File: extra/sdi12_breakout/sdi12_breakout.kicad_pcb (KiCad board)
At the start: 2 copper layers, 69 x 69 mm, 8 parts, among them J1 Conn_01x03_Socket, J2 Conn_01x03_Socket, J3 Conn_01x03_Socket, J4 Conn_01x03_Socket, J5 AudioJack3, J6 AudioJack3, J7 AudioJack3, J8 AudioJack3

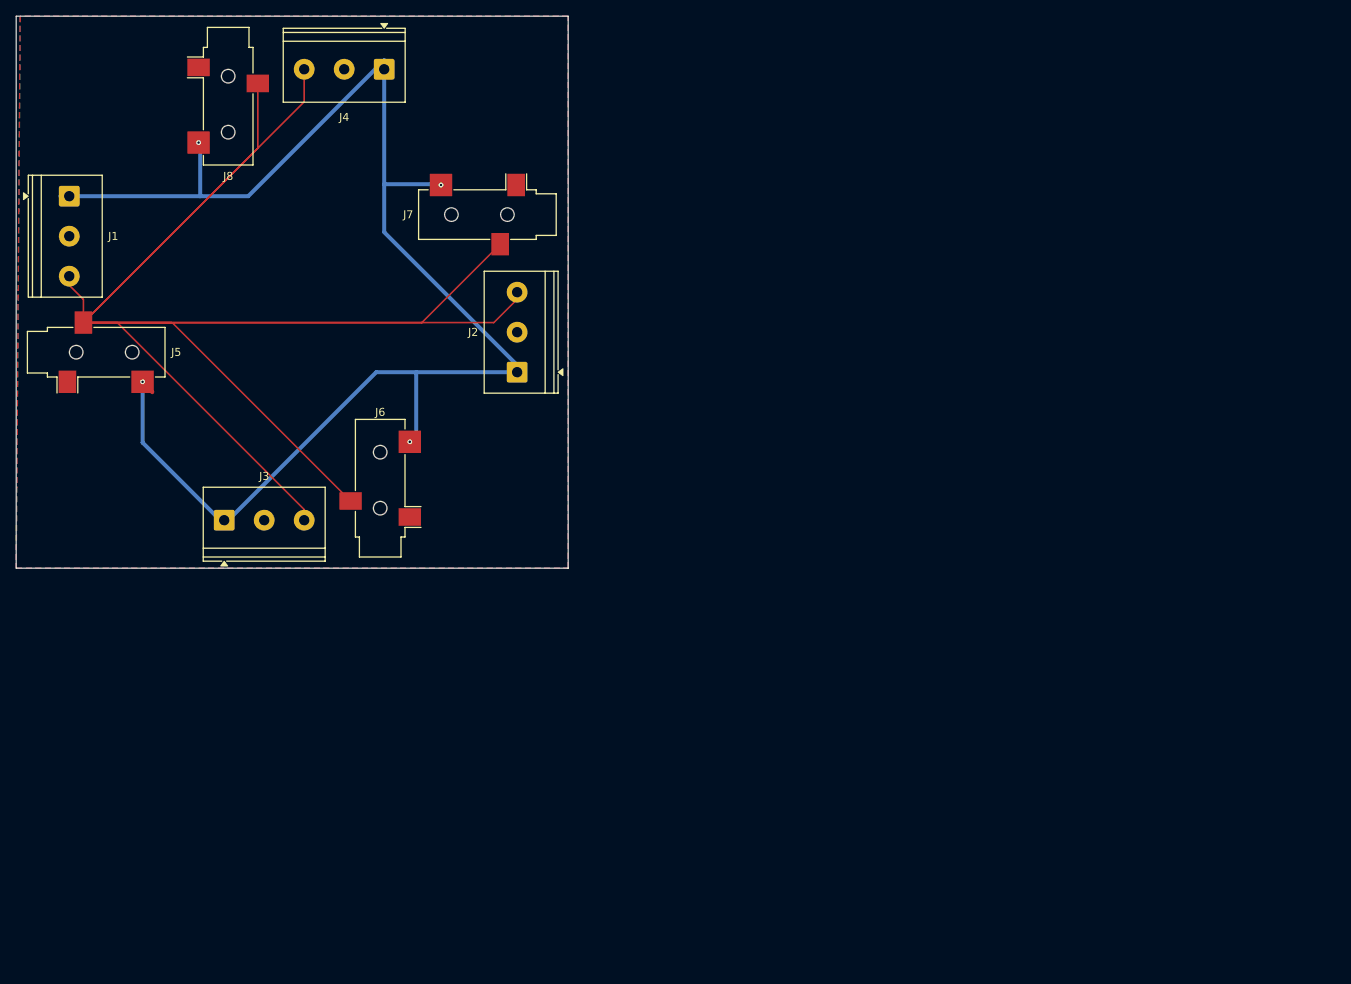
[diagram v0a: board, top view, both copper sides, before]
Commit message: Regenerated production file
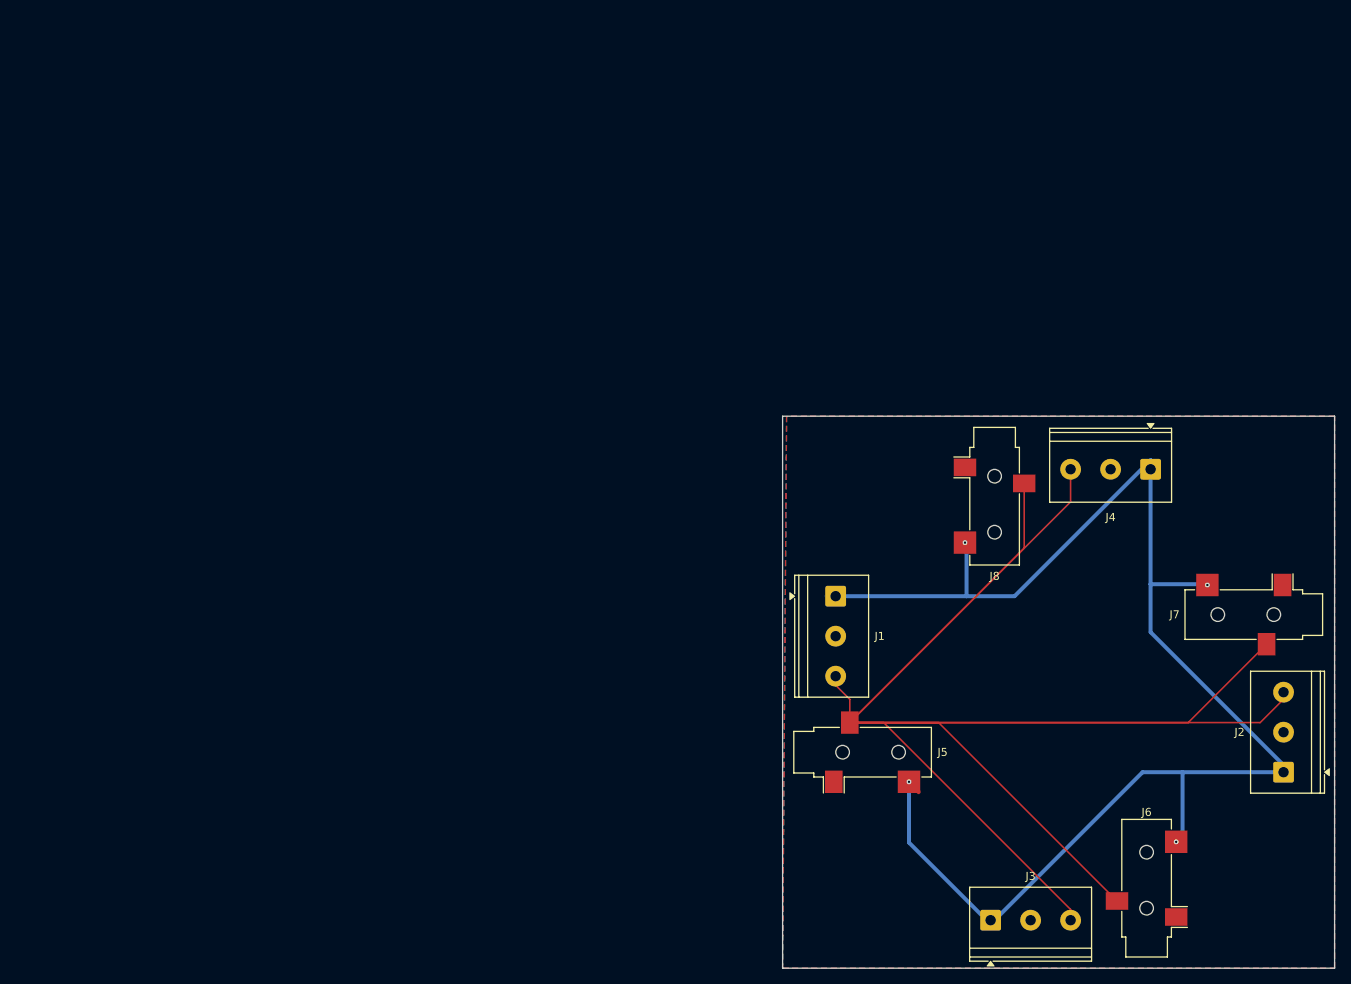
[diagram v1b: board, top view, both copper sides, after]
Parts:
- moved J1 108.1 mm to (114.9, 85.5)
- moved J3 108.1 mm to (134.3, 126.0)
- moved J4 108.1 mm to (154.3, 69.6)
- moved J6 108.1 mm to (153.8, 122.0)
- moved J8 108.1 mm to (134.8, 73.0)
- moved J5 108.1 mm to (118.3, 105.0)
- moved J2 108.1 mm to (170.9, 107.5)
- moved J7 108.1 mm to (167.2, 87.8)
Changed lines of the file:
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@@
 	(footprint "TerminalBlock_Phoenix:TerminalBlock_Phoenix_PT-1,5-3-5.0-H_1x03_P5.00mm_Horizontal"
 		(layer "F.Cu")
-		(at 75.1175 57.5 90)
+		(at 170.9175 107.5 90)
 		(descr "Terminal Block Phoenix PT-1,5-3-5.0-H, 3 pins, pitch 5mm, size 15x9mm, drill diameter 1.3mm, pad diameter 2.6mm, http://www.mouser.com/ds/2/324/ItemDetail_1935161-922578.pdf, script-generated using https://gitlab.com/kicad/libraries/kicad-footprint-generator/-/tree/master/scripts/TerminalBlock_Phoenix")
 		(tags "THT Terminal Block Phoenix PT-1,5-3-5.0-H pitch 5mm size 15x9mm drill 1.3mm pad 2.6mm")
@@
 	(footprint "TerminalBlock_Phoenix:TerminalBlock_Phoenix_PT-1,5-3-5.0-H_1x03_P5.00mm_Horizontal"
 		(layer "F.Cu")
-		(at 58.5 19.6325 180)
+		(at 154.3 69.6325 180)
 		(descr "Terminal Block Phoenix PT-1,5-3-5.0-H, 3 pins, pitch 5mm, size 15x9mm, drill diameter 1.3mm, pad diameter 2.6mm, http://www.mouser.com/ds/2/324/ItemDetail_1935161-922578.pdf, script-generated using https://gitlab.com/kicad/libraries/kicad-footprint-generator/-/tree/master/scripts/TerminalBlock_Phoenix")
 		(tags "THT Terminal Block Phoenix PT-1,5-3-5.0-H pitch 5mm size 15x9mm drill 1.3mm pad 2.6mm")
@@
 	(footprint "Connector_Audio:Jack_3.5mm_CUI_SJ-3523-SMT_Horizontal"
 		(layer "F.Cu")
-		(at 71.4 37.8 -90)
+		(at 167.2 87.8 -90)
 		(descr "3.5 mm, Stereo, Right Angle, Surface Mount (SMT), Audio Jack Connector (https://www.cui.com/product/resource/sj-352x-smt-series.pdf)")
 		(tags "3.5mm audio cui horizontal jack stereo")
@@
 	(footprint "Connector_Audio:Jack_3.5mm_CUI_SJ-3523-SMT_Horizontal"
 		(layer "F.Cu")
-		(at 22.5 55 90)
+		(at 118.3 105 90)
 		(descr "3.5 mm, Stereo, Right Angle, Surface Mount (SMT), Audio Jack Connector (https://www.cui.com/product/resource/sj-352x-smt-series.pdf)")
 		(tags "3.5mm audio cui horizontal jack stereo")
@@
 	(footprint "TerminalBlock_Phoenix:TerminalBlock_Phoenix_PT-1,5-3-5.0-H_1x03_P5.00mm_Horizontal"
 		(layer "F.Cu")
-		(at 38.5 76)
+		(at 134.3 126)
 		(descr "Terminal Block Phoenix PT-1,5-3-5.0-H, 3 pins, pitch 5mm, size 15x9mm, drill diameter 1.3mm, pad diameter 2.6mm, http://www.mouser.com/ds/2/324/ItemDetail_1935161-922578.pdf, script-generated using https://gitlab.com/kicad/libraries/kicad-footprint-generator/-/tree/master/scripts/TerminalBlock_Phoenix")
 		(tags "THT Terminal Block Phoenix PT-1,5-3-5.0-H pitch 5mm size 15x9mm drill 1.3mm pad 2.6mm")
@@
 	(footprint "Connector_Audio:Jack_3.5mm_CUI_SJ-3523-SMT_Horizontal"
 		(layer "F.Cu")
-		(at 58 72 180)
+		(at 153.8 122 180)
 		(descr "3.5 mm, Stereo, Right Angle, Surface Mount (SMT), Audio Jack Connector (https://www.cui.com/product/resource/sj-352x-smt-series.pdf)")
 		(tags "3.5mm audio cui horizontal jack stereo")
@@
 	(footprint "Connector_Audio:Jack_3.5mm_CUI_SJ-3523-SMT_Horizontal"
 		(layer "F.Cu")
-		(at 39 23)
+		(at 134.8 73)
 		(descr "3.5 mm, Stereo, Right Angle, Surface Mount (SMT), Audio Jack Connector (https://www.cui.com/product/resource/sj-352x-smt-series.pdf)")
 		(tags "3.5mm audio cui horizontal jack stereo")
@@
 	(footprint "TerminalBlock_Phoenix:TerminalBlock_Phoenix_PT-1,5-3-5.0-H_1x03_P5.00mm_Horizontal"
 		(layer "F.Cu")
-		(at 19.1325 35.5 -90)
+		(at 114.9325 85.5 -90)
 		(descr "Terminal Block Phoenix PT-1,5-3-5.0-H, 3 pins, pitch 5mm, size 15x9mm, drill diameter 1.3mm, pad diameter 2.6mm, http://www.mouser.com/ds/2/324/ItemDetail_1935161-922578.pdf, script-generated using https://gitlab.com/kicad/libraries/kicad-footprint-generator/-/tree/master/scripts/TerminalBlock_Phoenix")
 		(tags "THT Terminal Block Phoenix PT-1,5-3-5.0-H pitch 5mm size 15x9mm drill 1.3mm pad 2.6mm")
@@
 	)
 	(gr_rect
-		(start 12.5 13)
-		(end 81.5 82)
+		(start 108.3 63)
+		(end 177.3 132)
 		(stroke
 			(width 0.05)
@@
 	)
 	(gr_text "${TITLE}\n${COMPANY}\n${ISSUE_DATE}\n${REVISION}"
-		(at 56 50 0)
+		(at 151.8 100 0)
 		(layer "B.SilkS")
 		(effects
@@
 	)
 	(segment
-		(start 20.9 51.3)
-		(end 25.138477 51.3)
+		(start 116.7 101.3)
+		(end 120.938477 101.3)
 		(width 0.2)
 		(layer "F.Cu")
@@
 	)
 	(segment
-		(start 72.2 51.3)
-		(end 76 47.5)
+		(start 168 101.3)
+		(end 171.8 97.5)
 		(width 0.2)
 		(layer "F.Cu")
@@
 	)
 	(segment
-		(start 48.5 74.661523)
-		(end 48.5 76.5)
+		(start 144.3 124.661523)
+		(end 144.3 126.5)
 		(width 0.2)
 		(layer "F.Cu")
@@
 	)
 	(segment
-		(start 20.9 48.4)
-		(end 20.9 51.3)
+		(start 116.7 98.4)
+		(end 116.7 101.3)
 		(width 0.2)
 		(layer "F.Cu")
@@
 	)
 	(segment
-		(start 20.9 51.3)
-		(end 48.5 23.7)
+		(start 116.7 101.3)
+		(end 144.3 73.7)
 		(width 0.2)
 		(layer "F.Cu")
@@
 	)
 	(segment
-		(start 20.9 51.3)
-		(end 63.2 51.3)
+		(start 116.7 101.3)
+		(end 159 101.3)
 		(width 0.2)
 		(layer "F.Cu")
@@
 	)
 	(segment
-		(start 20.9 51.3)
-		(end 32 51.3)
+		(start 116.7 101.3)
+		(end 127.8 101.3)
 		(width 0.2)
 		(layer "F.Cu")
@@
 	)
 	(segment
-		(start 20.9 51.3)
-		(end 72.2 51.3)
+		(start 116.7 101.3)
+		(end 168 101.3)
 		(width 0.2)
 		(layer "F.Cu")
@@
 	)
 	(segment
-		(start 25.138477 51.3)
-		(end 48.5 74.661523)
+		(start 120.938477 101.3)
+		(end 144.3 124.661523)
 		(width 0.2)
 		(layer "F.Cu")
@@
 	)
 	(segment
-		(start 18 45.5)
-		(end 20.9 48.4)
+		(start 113.8 95.5)
+		(end 116.7 98.4)
 		(width 0.2)
 		(layer "F.Cu")
@@
 	)
 	(segment
-		(start 20.9 51.3)
-		(end 42.7 29.5)
+		(start 116.7 101.3)
+		(end 138.5 79.5)
 		(width 0.2)
 		(layer "F.Cu")
@@
 	)
 	(segment
-		(start 42.7 29.5)
-		(end 42.7 21.4)
+		(start 138.5 79.5)
+		(end 138.5 71.4)
 		(width 0.2)
 		(layer "F.Cu")
@@
 	)
 	(segment
-		(start 48.5 23.7)
-		(end 48.5 18.5)
+		(start 144.3 73.7)
+		(end 144.3 68.5)
 		(width 0.2)
 		(layer "F.Cu")
@@
 	)
 	(segment
-		(start 63.2 51.3)
-		(end 73 41.5)
+		(start 159 101.3)
+		(end 168.8 91.5)
 		(width 0.2)
 		(layer "F.Cu")
@@
 	)
 	(segment
-		(start 32 51.3)
-		(end 54.3 73.6)
+		(start 127.8 101.3)
+		(end 150.1 123.6)
 		(width 0.2)
 		(layer "F.Cu")
@@
 	)
 	(segment
-		(start 29.5 59.9)
-		(end 29.5 60)
+		(start 125.3 109.9)
+		(end 125.3 110)
 		(width 0.5)
 		(layer "F.Cu")
@@
 	)
 	(via
-		(at 65.6 34.1)
+		(at 161.4 84.1)
 		(size 0.6)
 		(drill 0.3)
@@
 	)
 	(via
-		(at 61.7 66.2)
+		(at 157.5 116.2)
 		(size 0.6)
 		(drill 0.3)
@@
 	)
 	(via
-		(at 35.3 28.8)
+		(at 131.1 78.8)
 		(size 0.6)
 		(drill 0.3)
@@
 	)
 	(via
-		(at 28.3 58.7)
+		(at 124.1 108.7)
 		(size 0.6)
 		(drill 0.3)
@@
 	)
 	(segment
-		(start 57.5 57.5)
-		(end 62.5 57.5)
+		(start 153.3 107.5)
+		(end 158.3 107.5)
 		(width 0.5)
 		(layer "B.Cu")
@@
 	)
 	(segment
-		(start 62.5 65.4)
-		(end 61.7 66.2)
+		(start 158.3 115.4)
+		(end 157.5 116.2)
 		(width 0.5)
 		(layer "B.Cu")
@@
 	)
 	(segment
-		(start 62.5 57.5)
-		(end 76 57.5)
+		(start 158.3 107.5)
+		(end 171.8 107.5)
 		(width 0.5)
 		(layer "B.Cu")
@@
 	)
 	(segment
-		(start 28.3 58.7)
-		(end 28.3 66.3)
+		(start 124.1 108.7)
+		(end 124.1 116.3)
 		(width 0.5)
 		(layer "B.Cu")
@@
 	)
 	(segment
-		(start 41.5 35.5)
-		(end 35.5 35.5)
+		(start 137.3 85.5)
+		(end 131.3 85.5)
 		(width 0.5)
 		(layer "B.Cu")
@@
 	)
 	(segment
-		(start 58.5 18.5)
-		(end 41.5 35.5)
+		(start 154.3 68.5)
+		(end 137.3 85.5)
 		(width 0.5)
 		(layer "B.Cu")
@@
 	)
 	(segment
-		(start 38.5 76.5)
-		(end 57.5 57.5)
+		(start 134.3 126.5)
+		(end 153.3 107.5)
 		(width 0.5)
 		(layer "B.Cu")
@@
 	)
 	(segment
-		(start 58.5 40)
-		(end 58.5 34)
+		(start 154.3 90)
+		(end 154.3 84)
 		(width 0.5)
 		(layer "B.Cu")
@@
 	)
 	(segment
-		(start 58.5 34)
-		(end 58.5 18.5)
+		(start 154.3 84)
+		(end 154.3 68.5)
 		(width 0.5)
 		(layer "B.Cu")
@@
 	)
 	(segment
-		(start 58.5 34)
-		(end 65.5 34)
+		(start 154.3 84)
+		(end 161.3 84)
 		(width 0.5)
 		(layer "B.Cu")
@@
 	)
 	(segment
-		(start 35.5 35.5)
-		(end 35.5 29)
+		(start 131.3 85.5)
+		(end 131.3 79)
 		(width 0.5)
 		(layer "B.Cu")
@@
 	)
 	(segment
-		(start 28.3 66.3)
-		(end 38.5 76.5)
+		(start 124.1 116.3)
+		(end 134.3 126.5)
 		(width 0.5)
 		(layer "B.Cu")
@@
 	)
 	(segment
-		(start 35.5 29)
-		(end 35.3 28.8)
+		(start 131.3 79)
+		(end 131.1 78.8)
 		(width 0.5)
 		(layer "B.Cu")
@@
 	)
 	(segment
-		(start 65.5 34)
-		(end 65.6 34.1)
+		(start 161.3 84)
+		(end 161.4 84.1)
 		(width 0.5)
 		(layer "B.Cu")
@@
 	)
 	(segment
-		(start 76 57.5)
-		(end 58.5 40)
+		(start 171.8 107.5)
+		(end 154.3 90)
 		(width 0.5)
 		(layer "B.Cu")
@@
 	)
 	(segment
-		(start 35.5 35.5)
-		(end 18 35.5)
+		(start 131.3 85.5)
+		(end 113.8 85.5)
 		(width 0.5)
 		(layer "B.Cu")
@@
 	)
 	(segment
-		(start 62.5 57.5)
-		(end 62.5 65.4)
+		(start 158.3 107.5)
+		(end 158.3 115.4)
 		(width 0.5)
 		(layer "B.Cu")
@@
 		(polygon
 			(pts
-				(xy 81.5 13) (xy 13 13) (xy 12.5 82) (xy 81.5 82)
+				(xy 177.3 63) (xy 108.8 63) (xy 108.3 132) (xy 177.3 132)
 			)
 		)
